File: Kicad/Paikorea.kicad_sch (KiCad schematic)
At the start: 49 parts, among them J1 AudioJack3, J2 TPS43-201A-S, J4 AudioJack3, K10 PG1316S, K11 PG1316S, K12 PG1316S, K13 PG1316S, K14 PG1316S, K15 PG1316S, K16 PG1316S, K17 PG1316S, K18 PG1316S, K19 PG1316S, K20 PG1316S, K21 PG1316S, K22 PG1316S, K4 PG1316S, K5 PG1316S, K6 PG1316S, K7 PG1316S, K8 PG1316S, K9 PG1316S, U1 RP2040-Zero, U2 RP2040-Zero

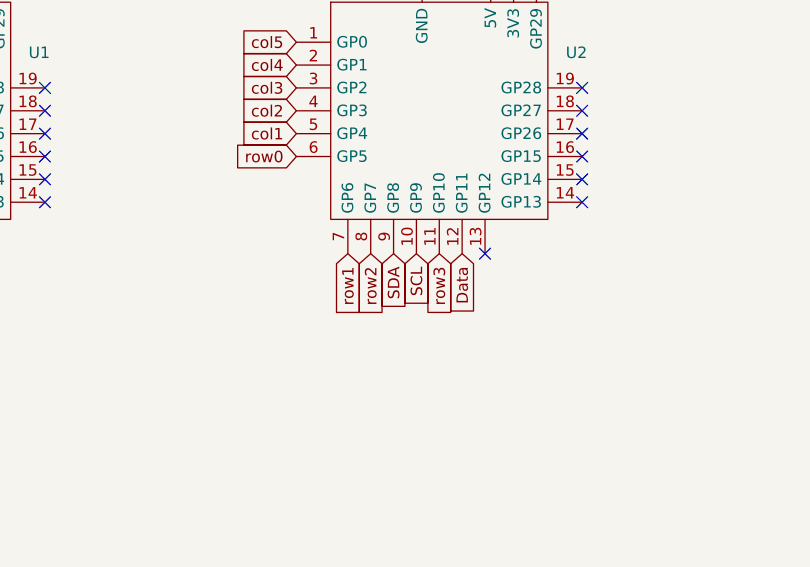
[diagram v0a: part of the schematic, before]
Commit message: .
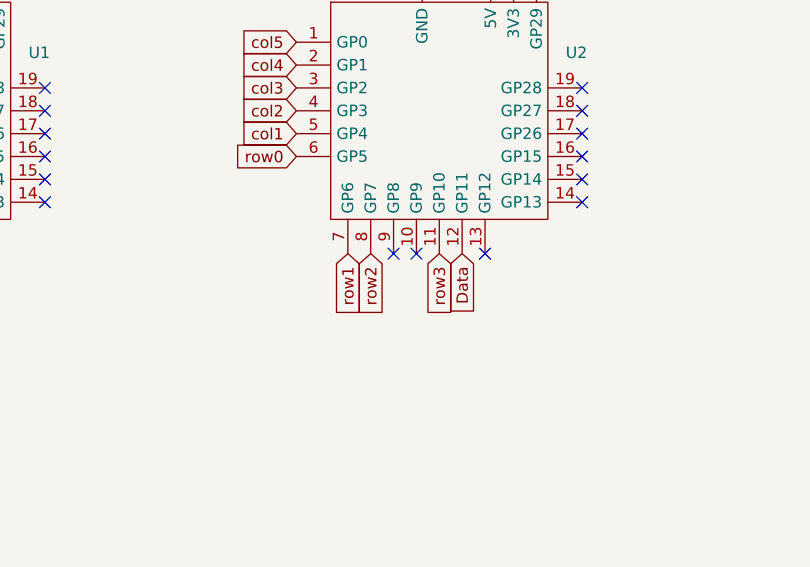
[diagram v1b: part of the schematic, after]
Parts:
- J1, J4: footprint DreaM117er-keebLibrary:TRRS-PJ-381-BB_6P_Dual -> Connector_Audio:Jack_3.5mm_KoreanHropartsElec_PJ-320D-4A_Horizontal
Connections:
- net SCL: no longer U2.10 (GP9)
- net SDA: no longer U2.9 (GP8)
- no-connect marks 18 -> 20

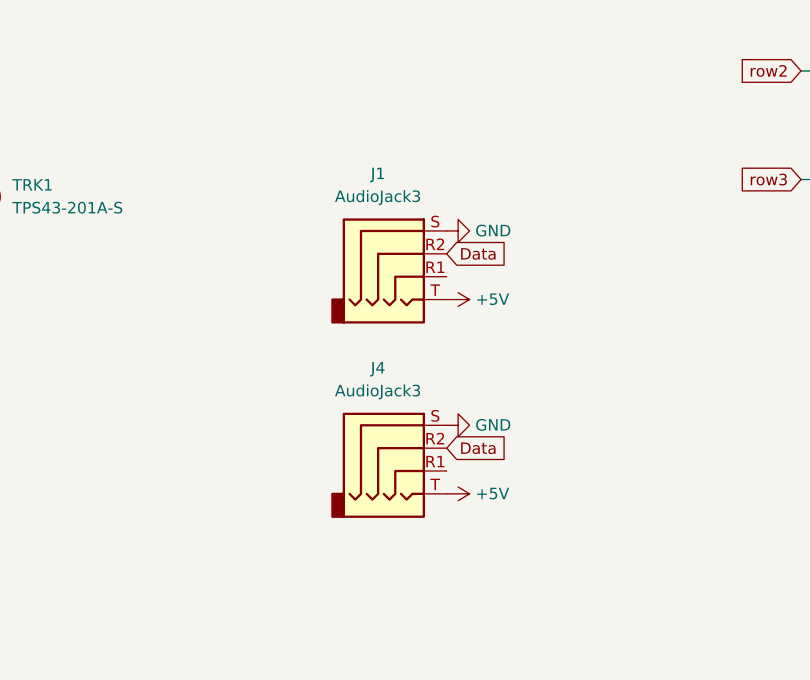
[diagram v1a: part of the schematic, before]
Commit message: .
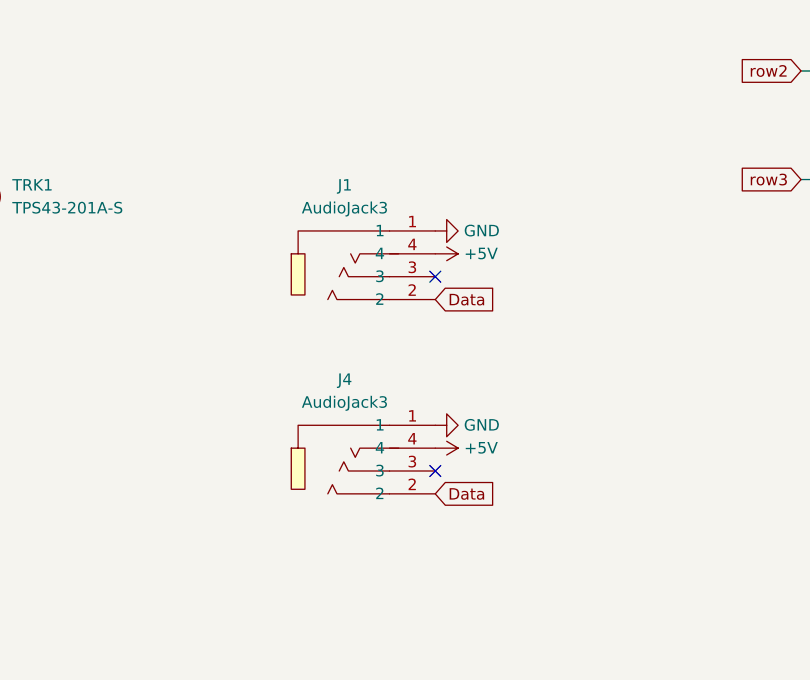
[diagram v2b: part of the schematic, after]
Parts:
- J1, J4: footprint Connector_Audio:Jack_3.5mm_KoreanHropartsElec_PJ-320D-4A_Horizontal -> Paikorea:AUDIO-SMD_PJ-320D-1; symbol Connector_Audio:AudioJack4 -> Paikorea:PJ-320D; LCSC Part (none) -> C431535; MPN (none) -> PJ-320D; Manufacturer (none) -> SHOU HAN(首韩)
- U1, U2: footprint Paikorea:RP2040-Zero_UpsideDown -> Paikorea:RP2040-Zero-smd
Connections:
- net +5V: now also J1.4, J4.4; no longer J1.T, J4.T
- net Data: now also J1.2, J4.2; no longer J1.R2, J4.R2
- net GND: now also J1.1, J4.1; no longer J1.S, J4.S
- no-connect marks 20 -> 22
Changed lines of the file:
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@@
 	)
 	(no_connect
+		(at 232.41 106.68)
+	)
+	(no_connect
 		(at 78.105 120.015)
 	)
@@
 	)
 	(no_connect
+		(at 232.41 128.27)
+	)
+	(no_connect
 		(at 142.875 135.89)
 	)
@@
 	(global_label "Data"
 		(shape input)
-		(at 233.68 125.73 0)
+		(at 232.41 130.81 0)
 		(fields_autoplaced yes)
 		(effects
@@
 		)
 		(property "Intersheetrefs" "${INTERSHEET_REFS}"
-			(at 240.8795 125.73 0)
+			(at 239.6095 130.81 0)
 			(hide yes)
 			(show_name no)
@@
 	(global_label "Data"
 		(shape input)
-		(at 233.68 104.14 0)
+		(at 232.41 109.22 0)
 		(fields_autoplaced yes)
 		(effects
@@
 		)
 		(property "Intersheetrefs" "${INTERSHEET_REFS}"
-			(at 240.8795 104.14 0)
+			(at 239.6095 109.22 0)
 			(hide yes)
 			(show_name no)
@@
 	(symbol
 		(lib_id "power:+5V")
-		(at 233.68 109.22 270)
+		(at 232.41 104.14 270)
 		(unit 1)
 		(body_style 1)
@@
 		(dnp no)
 		(property "Reference" "#PWR037"
-			(at 229.87 109.22 0)
+			(at 228.6 104.14 0)
 			(hide yes)
 			(show_name no)
@@
 		)
 		(property "Value" "+5V"
-			(at 238.76 109.22 90)
+			(at 237.49 104.14 90)
 			(show_name no)
 			(do_not_autoplace no)
@@
 		)
 		(property "Footprint" ""
-			(at 233.68 109.22 0)
+			(at 232.41 104.14 0)
 			(hide yes)
 			(show_name no)
@@
 		)
 		(property "Datasheet" ""
-			(at 233.68 109.22 0)
+			(at 232.41 104.14 0)
 			(hide yes)
 			(show_name no)
@@
 		)
 		(property "Description" ""
-			(at 233.68 109.22 0)
+			(at 232.41 104.14 0)
 			(show_name no)
 			(do_not_autoplace no)
@@
 	)
 	(symbol
-		(lib_id "Connector_Audio:AudioJack4")
-		(at 228.6 125.73 0)
+		(lib_id "Paikorea:PJ-320D")
+		(at 224.79 125.73 0)
 		(unit 1)
 		(body_style 1)
@@
 		(fields_autoplaced yes)
 		(property "Reference" "J4"
-			(at 226.06 116.84 0)
+			(at 222.38 118.11 0)
 			(show_name no)
 			(do_not_autoplace no)
@@
 		)
 		(property "Value" "AudioJack3"
-			(at 226.06 119.38 0)
+			(at 222.38 120.65 0)
 			(show_name no)
 			(do_not_autoplace no)
@@
 			)
 		)
-		(property "Footprint" "Connector_Audio:Jack_3.5mm_KoreanHropartsElec_PJ-320D-4A_Horizontal"
-			(at 228.6 125.73 0)
+		(property "Footprint" "Paikorea:AUDIO-SMD_PJ-320D-1"
+			(at 224.79 138.43 0)
 			(hide yes)
 			(show_name no)
@@
 			)
 		)
-		(property "Datasheet" ""
-			(at 228.6 125.73 0)
+		(property "Datasheet" "https://lcsc.com/product-detail/Audio-Video-Connectors_SHOU-HAN-PJ-320D_C431535.html"
+			(at 224.79 140.97 0)
 			(hide yes)
 			(show_name no)
@@
 		)
 		(property "Description" "Audio Jack, 4 Poles (TRRS)"
-			(at 228.6 125.73 0)
+			(at 224.79 125.73 0)
+			(hide yes)
+			(show_name no)
+			(do_not_autoplace no)
+			(effects
+				(font
+					(size 1.27 1.27)
+				)
+			)
+		)
+		(property "Manufacturer" "SHOU HAN(首韩)"
+			(at 224.79 143.51 0)
+			(hide yes)
+			(show_name no)
+			(do_not_autoplace no)
+			(effects
+				(font
+					(size 1.27 1.27)
+				)
+			)
+		)
+		(property "MPN" "PJ-320D"
+			(at 224.79 146.05 0)
 			(hide yes)
 			(show_name no)
@@
 			)
 		)
-		(pin "R1"
+		(property "LCSC Part" "C431535"
+			(at 224.79 148.59 0)
+			(hide yes)
+			(show_name no)
+			(do_not_autoplace no)
+			(effects
+				(font
+					(size 1.27 1.27)
+				)
+			)
+		)
+		(pin "1"
 		)
-		(pin "S"
+		(pin "3"
 		)
-		(pin "T"
+		(pin "4"
 		)
-		(pin "R2"
+		(pin "2"
 		)
 		(instances
@@
 	(symbol
 		(lib_id "power:GND")
-		(at 233.68 101.6 90)
+		(at 232.41 101.6 90)
 		(unit 1)
 		(body_style 1)
@@
 		(dnp no)
 		(property "Reference" "#PWR036"
-			(at 240.03 101.6 0)
+			(at 238.76 101.6 0)
 			(hide yes)
 			(show_name no)
@@
 		)
 		(property "Value" "GND"
-			(at 236.855 101.6 90)
+			(at 235.585 101.6 90)
 			(show_name no)
 			(do_not_autoplace no)
@@
 		)
 		(property "Footprint" ""
-			(at 233.68 101.6 0)
+			(at 232.41 101.6 0)
 			(hide yes)
 			(show_name no)
@@
 		)
 		(property "Datasheet" ""
-			(at 233.68 101.6 0)
+			(at 232.41 101.6 0)
 			(hide yes)
 			(show_name no)
@@
 		)
 		(property "Description" ""
-			(at 233.68 101.6 0)
+			(at 232.41 101.6 0)
 			(show_name no)
 			(do_not_autoplace no)
@@
 			)
 		)
-		(property "Footprint" "Paikorea:RP2040-Zero_UpsideDown"
+		(property "Footprint" "Paikorea:RP2040-Zero-smd"
 			(at 150.495 137.795 90)
 			(hide yes)
@@
 	)
 	(symbol
-		(lib_id "Connector_Audio:AudioJack4")
-		(at 228.6 104.14 0)
+		(lib_id "Paikorea:PJ-320D")
+		(at 224.79 104.14 0)
 		(unit 1)
 		(body_style 1)
@@
 		(fields_autoplaced yes)
 		(property "Reference" "J1"
-			(at 226.06 95.25 0)
+			(at 222.38 96.52 0)
 			(show_name no)
 			(do_not_autoplace no)
@@
 		)
 		(property "Value" "AudioJack3"
-			(at 226.06 97.79 0)
+			(at 222.38 99.06 0)
 			(show_name no)
 			(do_not_autoplace no)
@@
 			)
 		)
-		(property "Footprint" "Connector_Audio:Jack_3.5mm_KoreanHropartsElec_PJ-320D-4A_Horizontal"
-			(at 228.6 104.14 0)
+		(property "Footprint" "Paikorea:AUDIO-SMD_PJ-320D-1"
+			(at 224.79 116.84 0)
 			(hide yes)
 			(show_name no)
@@
 			)
 		)
-		(property "Datasheet" ""
-			(at 228.6 104.14 0)
+		(property "Datasheet" "https://lcsc.com/product-detail/Audio-Video-Connectors_SHOU-HAN-PJ-320D_C431535.html"
+			(at 224.79 119.38 0)
 			(hide yes)
 			(show_name no)
@@
 		)
 		(property "Description" "Audio Jack, 4 Poles (TRRS)"
-			(at 228.6 104.14 0)
+			(at 224.79 104.14 0)
+			(hide yes)
+			(show_name no)
+			(do_not_autoplace no)
+			(effects
+				(font
+					(size 1.27 1.27)
+				)
+			)
+		)
+		(property "Manufacturer" "SHOU HAN(首韩)"
+			(at 224.79 121.92 0)
+			(hide yes)
+			(show_name no)
+			(do_not_autoplace no)
+			(effects
+				(font
+					(size 1.27 1.27)
+				)
+			)
+		)
+		(property "MPN" "PJ-320D"
+			(at 224.79 124.46 0)
 			(hide yes)
 			(show_name no)
@@
 			)
 		)
-		(pin "R1"
+		(property "LCSC Part" "C431535"
+			(at 224.79 127 0)
+			(hide yes)
+			(show_name no)
+			(do_not_autoplace no)
+			(effects
+				(font
+					(size 1.27 1.27)
+				)
+			)
 		)
-		(pin "S"
+		(pin "2"
 		)
-		(pin "T"
+		(pin "1"
 		)
-		(pin "R2"
+		(pin "3"
+		)
+		(pin "4"
 		)
 		(instances
@@
 			)
 		)
-		(property "Footprint" "Paikorea:RP2040-Zero_UpsideDown"
+		(property "Footprint" "Paikorea:RP2040-Zero-smd"
 			(at 90.805 137.795 90)
 			(hide yes)
@@
 	(symbol
 		(lib_id "power:GND")
-		(at 233.68 123.19 90)
+		(at 232.41 123.19 90)
 		(unit 1)
 		(body_style 1)
@@
 		(dnp no)
 		(property "Reference" "#PWR030"
-			(at 240.03 123.19 0)
+			(at 238.76 123.19 0)
 			(hide yes)
 			(show_name no)
@@
 		)
 		(property "Value" "GND"
-			(at 236.855 123.19 90)
+			(at 235.585 123.19 90)
 			(show_name no)
 			(do_not_autoplace no)
@@
 		)
 		(property "Footprint" ""
-			(at 233.68 123.19 0)
+			(at 232.41 123.19 0)
 			(hide yes)
 			(show_name no)
@@
 		)
 		(property "Datasheet" ""
-			(at 233.68 123.19 0)
+			(at 232.41 123.19 0)
 			(hide yes)
 			(show_name no)
@@
 		)
 		(property "Description" ""
-			(at 233.68 123.19 0)
+			(at 232.41 123.19 0)
 			(show_name no)
 			(do_not_autoplace no)
@@
 	(symbol
 		(lib_id "power:+5V")
-		(at 233.68 130.81 270)
+		(at 232.41 125.73 270)
 		(unit 1)
 		(body_style 1)
@@
 		(dnp no)
 		(property "Reference" "#PWR035"
-			(at 229.87 130.81 0)
+			(at 228.6 125.73 0)
 			(hide yes)
 			(show_name no)
@@
 		)
 		(property "Value" "+5V"
-			(at 238.76 130.81 90)
+			(at 237.49 125.73 90)
 			(show_name no)
 			(do_not_autoplace no)
@@
 		)
 		(property "Footprint" ""
-			(at 233.68 130.81 0)
+			(at 232.41 125.73 0)
 			(hide yes)
 			(show_name no)
@@
 		)
 		(property "Datasheet" ""
-			(at 233.68 130.81 0)
+			(at 232.41 125.73 0)
 			(hide yes)
 			(show_name no)
@@
 		)
 		(property "Description" ""
-			(at 233.68 130.81 0)
+			(at 232.41 125.73 0)
 			(show_name no)
 			(do_not_autoplace no)
